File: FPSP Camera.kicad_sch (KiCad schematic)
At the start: 77 parts, among them J1 USB_B_Micro, J2 Conn_02x06_Odd_Even, J3 SM03B-SRSS-TB, J4 Conn_01x24_Socket, U1 TLV75533PDRV, U2 TLV73328PDRV, U3 RP2350_60QFN, U4 TLV73315PDRV, U5 W25Q128JVS, U6 ICM-45686, Y1 SiT8008xx-1x-xxE

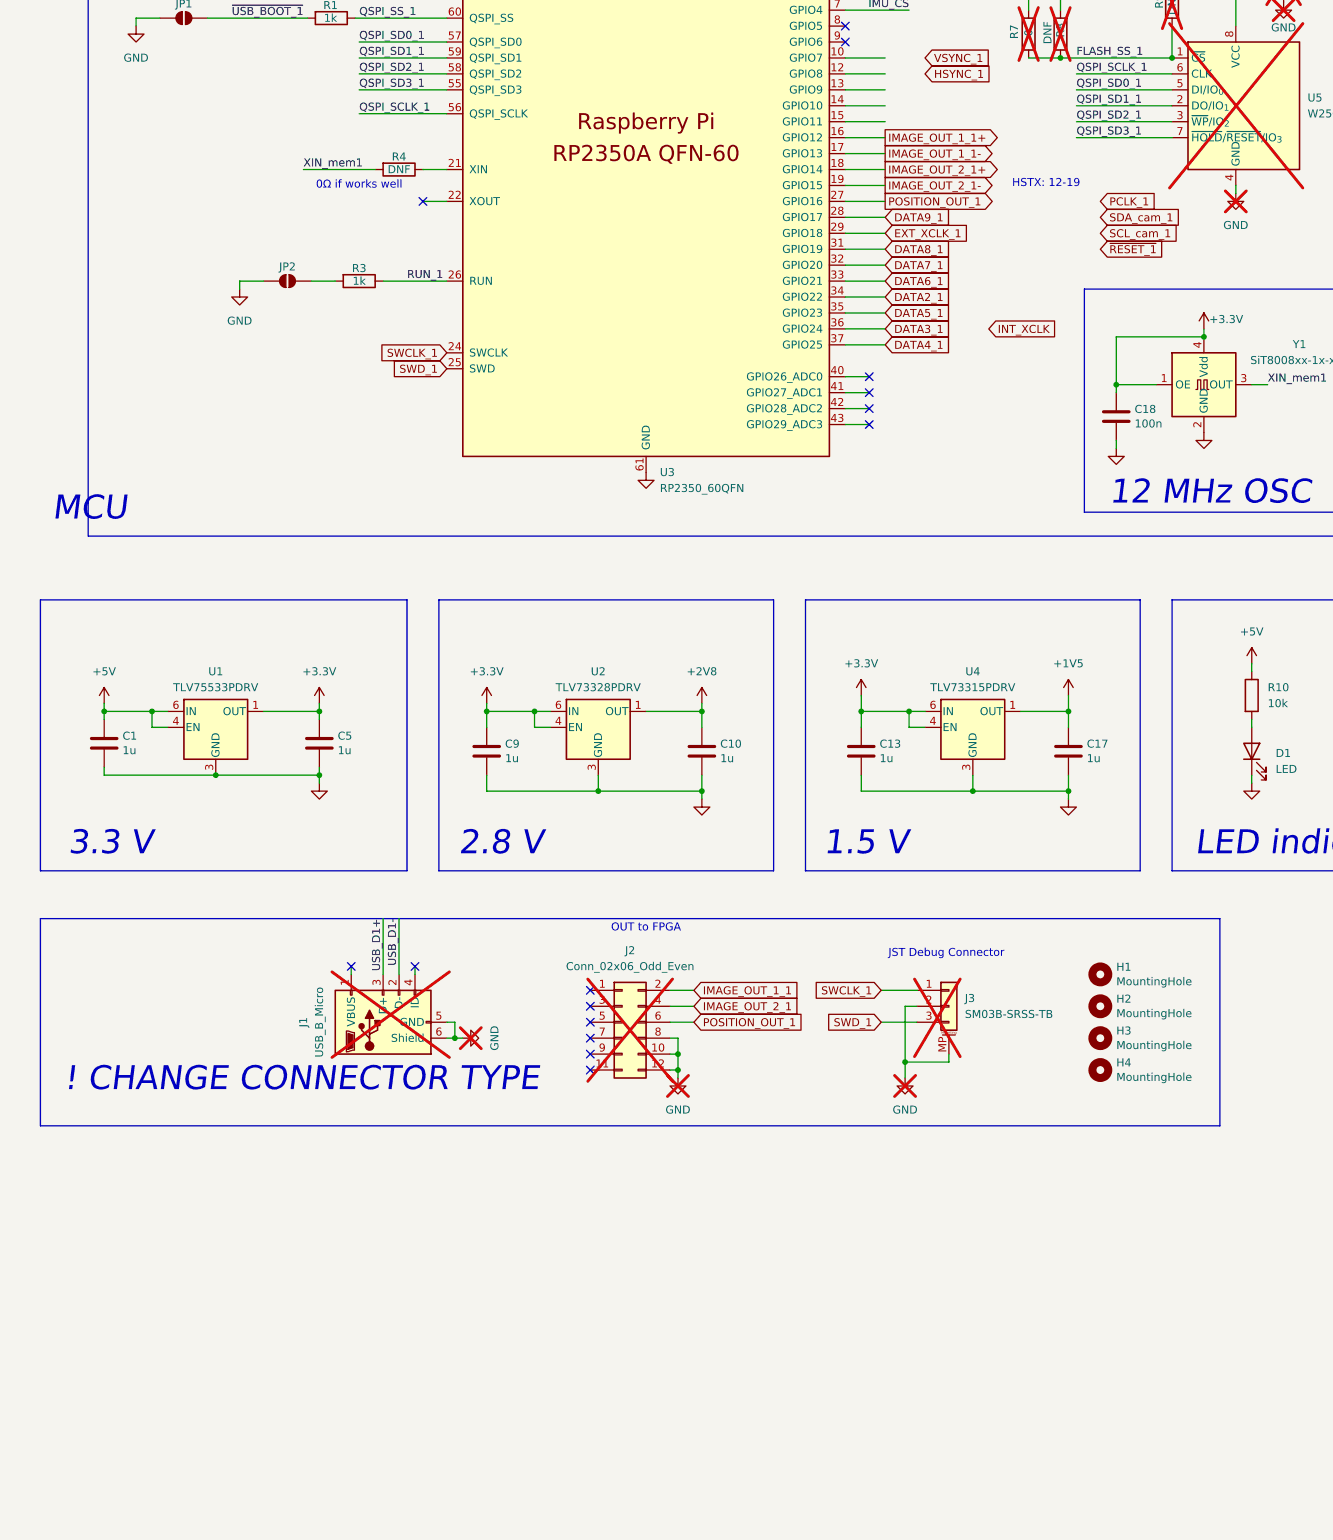
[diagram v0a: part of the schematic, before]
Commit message: connector PCB added
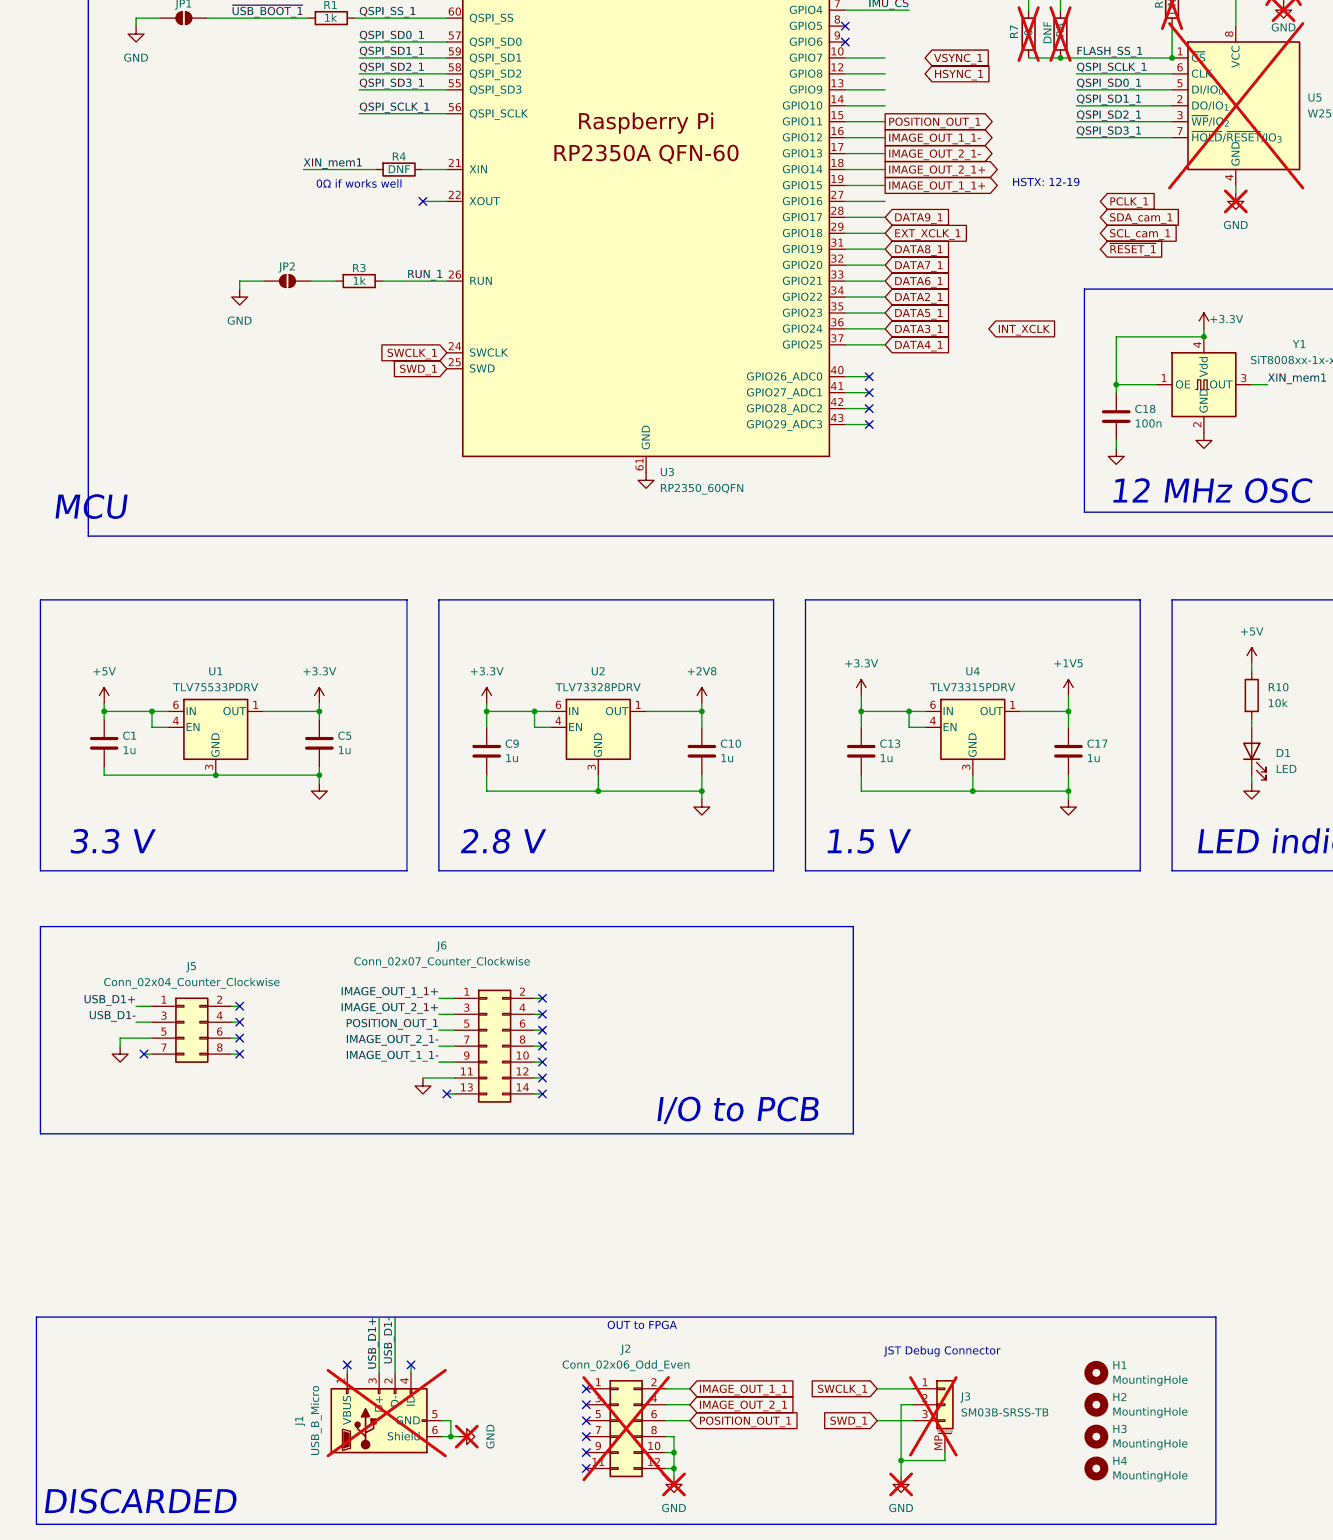
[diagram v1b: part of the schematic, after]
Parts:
- added J5: Conn_02x04_Counter_Clockwise, Connector_Molex:Molex_SlimStack_502426-0810_2x04_P0.40mm_Vertical, symbol Connector_Generic:Conn_02x04_Odd_Even
- added J6: Conn_02x07_Counter_Clockwise, Connector_Molex:Molex_SlimStack_502426-1410_2x07_P0.40mm_Vertical, symbol Connector_Generic:Conn_02x07_Odd_Even
- R10, R11, R12, R15: footprint Capacitor_SMD:C_0402_1005Metric -> Resistor_SMD:R_0603_1608Metric_Pad0.98x0.95mm_HandSolder
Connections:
- net GND: now also J5.5 (Pin_5), J6.11 (Pin_11)
- net IMAGE_OUT_1_1+: now also U3.19 (GPIO15), J6.1 (Pin_1); no longer U3.16 (GPIO12)
- net IMAGE_OUT_1_1-: now also U3.16 (GPIO12), J6.9 (Pin_9); no longer U3.17 (GPIO13)
- net IMAGE_OUT_2_1+: now also J6.3 (Pin_3)
- net IMAGE_OUT_2_1-: now also U3.17 (GPIO13), J6.7 (Pin_7); no longer U3.19 (GPIO15)
- net POSITION_OUT_1: now also U3.15 (GPIO11), J6.5 (Pin_5); no longer U3.27 (GPIO16)
- net USB_D1+: now also J5.1 (Pin_1)
- net USB_D1-: now also J5.3 (Pin_3)
- no-connect marks 23 -> 36
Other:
- note added: "DISCARDED"
- note added: "I/O to PCB"
- note removed: "! CHANGE CONNECTOR TYPE"
- moved on the sheet: H1, H2, H3, H4, J1, J2, J3
